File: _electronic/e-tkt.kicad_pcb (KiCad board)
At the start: 4 copper layers, 99.6 x 76.2 mm, 110 parts

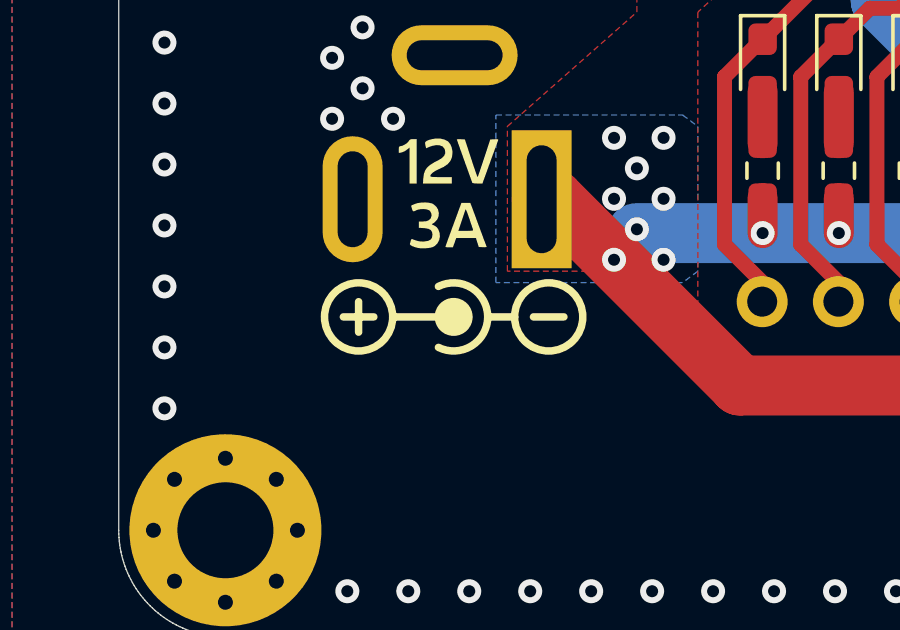
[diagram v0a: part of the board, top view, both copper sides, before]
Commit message: pcb v1 to production
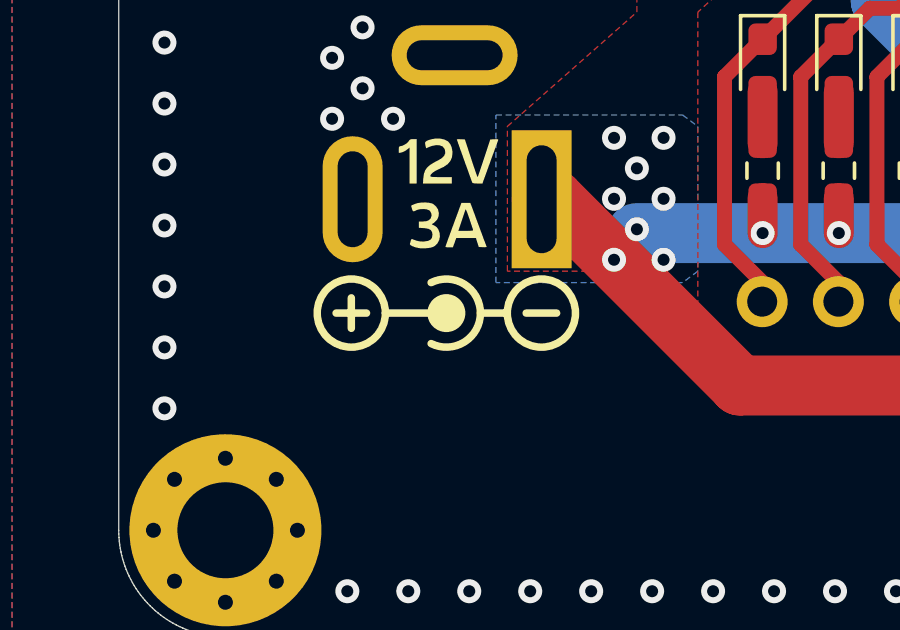
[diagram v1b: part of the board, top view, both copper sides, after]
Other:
- board text added: "2022/09/23"
- board text removed: "2022/09/21"
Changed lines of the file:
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@@
       (xy 149.352 -213.36)
     ) (layer "B.SilkS") (width 0.15) (fill solid))
-  (gr_line (start 144.379749 -162.052002) (end 145.27631 -162.052002) (layer "F.SilkS") (width 0.25))
-  (gr_circle (center 143.24431 -162.052002) (end 143.24431 -162.560002) (layer "F.SilkS") (width 0.25) (fill solid))
-  (gr_line (start 146.920232 -162.052002) (end 145.904232 -162.052002) (layer "F.SilkS") (width 0.25))
-  (gr_line (start 141.211827 -162.052002) (end 143.243976 -162.052002) (layer "F.SilkS") (width 0.25))
-  (gr_arc (start 142.73631 -163.068002) (mid 144.379784 -162.052002) (end 142.73631 -161.036002) (layer "F.SilkS") (width 0.25))
-  (gr_line (start 139.567905 -162.052002) (end 140.583905 -162.052002) (layer "F.SilkS") (width 0.25))
-  (gr_circle (center 146.412232 -162.052002) (end 146.412232 -163.187925) (layer "F.SilkS") (width 0.25) (fill none))
-  (gr_line (start 140.075905 -161.544002) (end 140.075905 -162.560002) (layer "F.SilkS") (width 0.25))
-  (gr_circle (center 140.075905 -162.052002) (end 140.075905 -163.187925) (layer "F.SilkS") (width 0.25) (fill none))
+  (gr_line (start 144.136437 -162.179) (end 145.032998 -162.179) (layer "F.SilkS") (width 0.25))
+  (gr_circle (center 143.000998 -162.179) (end 143.000998 -162.687) (layer "F.SilkS") (width 0.25) (fill solid))
+  (gr_line (start 146.67692 -162.179) (end 145.66092 -162.179) (layer "F.SilkS") (width 0.25))
+  (gr_line (start 140.968515 -162.179) (end 143.000664 -162.179) (layer "F.SilkS") (width 0.25))
+  (gr_arc (start 142.492998 -163.195) (mid 144.136474 -162.178997) (end 142.492998 -161.163) (layer "F.SilkS") (width 0.25))
+  (gr_line (start 139.324593 -162.179) (end 140.340593 -162.179) (layer "F.SilkS") (width 0.25))
+  (gr_circle (center 146.16892 -162.179) (end 146.16892 -163.314923) (layer "F.SilkS") (width 0.25) (fill none))
+  (gr_line (start 139.832593 -161.671) (end 139.832593 -162.687) (layer "F.SilkS") (width 0.25))
+  (gr_circle (center 139.832593 -162.179) (end 139.832593 -163.314923) (layer "F.SilkS") (width 0.25) (fill none))
   (gr_line (start 134.560258 -151.550617) (end 134.445168 -151.58932) (layer "Edge.Cuts") (width 0.02))
   (gr_line (start 131.831791 -178.139401) (end 131.785272 -178.251708) (layer "Edge.Cuts") (width 0.02))
@@
     (effects (font (size 2 2) (thickness 0.3)))
   )
-  (gr_text "2022/09/21" (at 139.7 -154.94) (layer "B.Mask")
+  (gr_text "2022/09/23" (at 139.7 -154.94) (layer "B.Mask")
     (effects (font (size 1.3 1.3) (thickness 0.3)) (justify right mirror))
   )
